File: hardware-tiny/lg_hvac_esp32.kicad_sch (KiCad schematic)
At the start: 16 parts, among them J1 JST_XH_S3B-XH-A-1_01x03, J2 Conn_01x19_Female_1_to_19, J3 Conn_01x19_Female_20_to_38, U1 TPS82130, U2 TJA1027

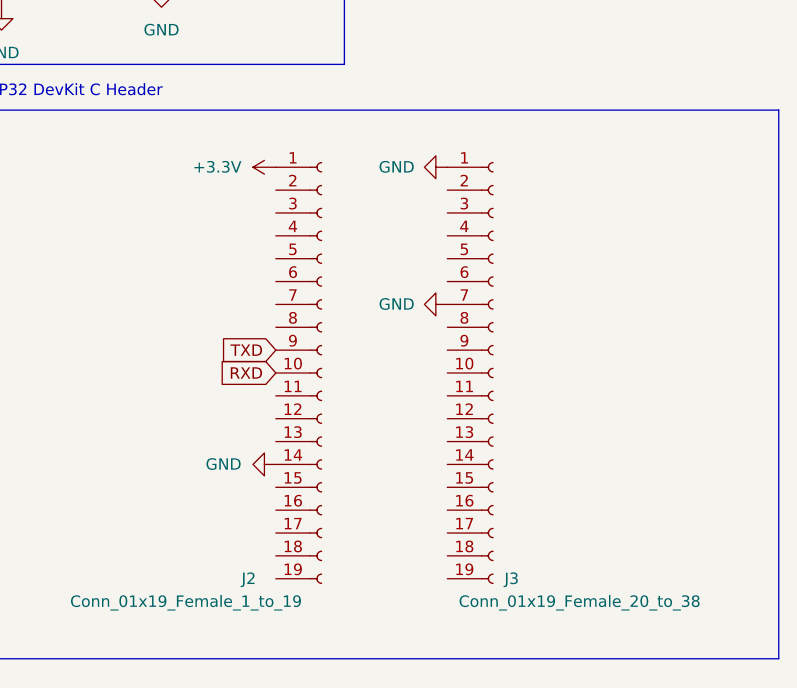
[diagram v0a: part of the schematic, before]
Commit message: fixed bom and updated kicad project to kicad7 #17
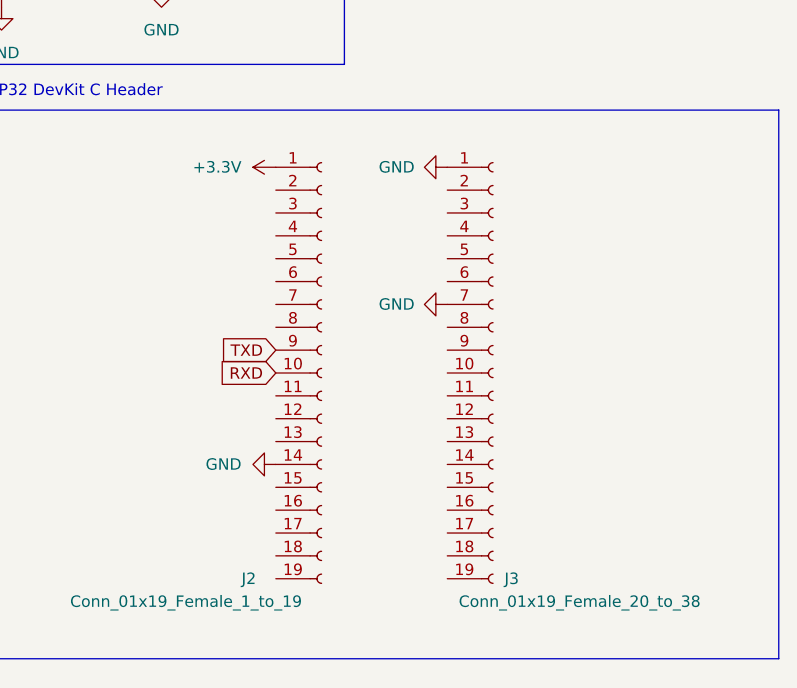
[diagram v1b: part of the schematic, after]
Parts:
- C2: LCSC C343058 -> C26404
- U1: footprint TPS82130:CONV_TPS82140SILR -> Package_LGA:Texas_MicroSiP-8-1EP_2.8x3.0mm_P0.65mm_EP1.1x1.9mm_SMD_ThermalVias
